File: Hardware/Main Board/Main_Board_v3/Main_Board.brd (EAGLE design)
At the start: 105.4 x 84.8 mm, 69 parts, among them IC1 MBED_MICROCONTROLLER, IC2 NE555, Q1 BS170, Q2 BS170, Q3 IRF3704L-V, Q4 IRF3704L-V, Q5 BS170, Q6 IRF3704L-V, Q7 BS170, Q8 IRF3704L-V

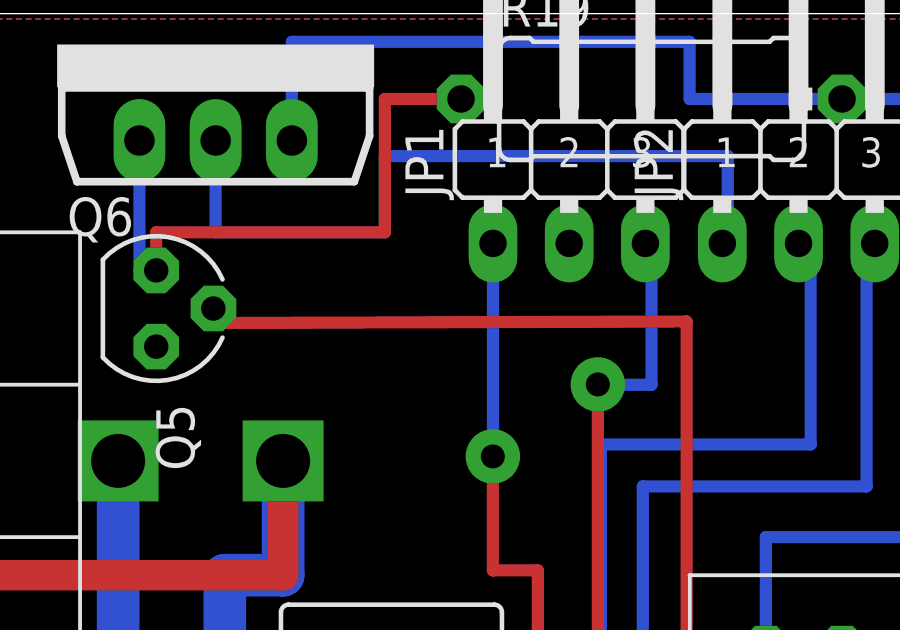
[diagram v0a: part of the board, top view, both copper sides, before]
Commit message: Board Layouts done for DC Current and AC Board
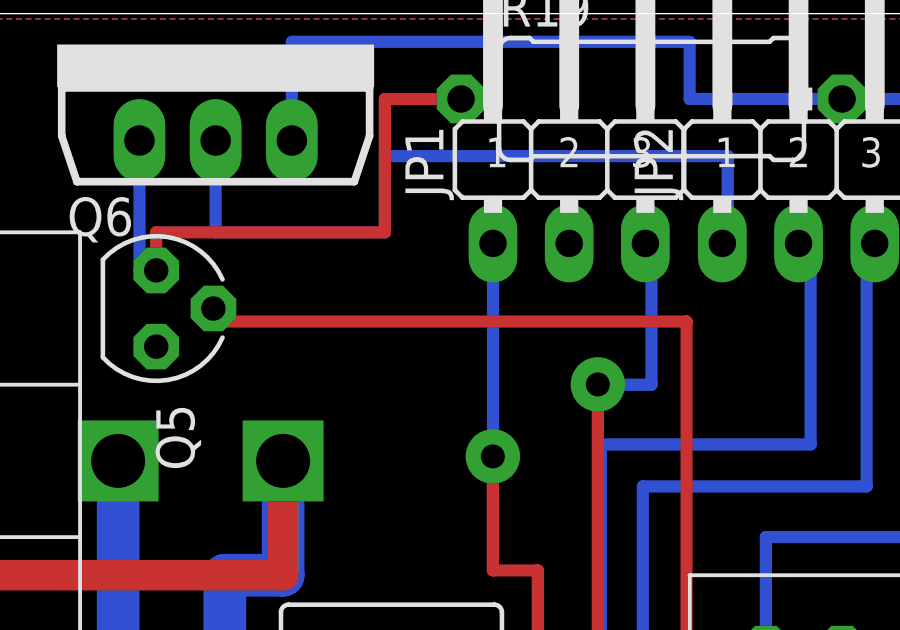
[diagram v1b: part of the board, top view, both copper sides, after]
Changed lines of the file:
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@@
 <wire x1="62.23" y1="53.34" x2="35.4584" y2="53.3908" width="0.4064" layer="1"/>
 <wire x1="35.4584" y1="53.3908" x2="35.4584" y2="74.4982" width="0.4064" layer="1"/>
-<wire x1="35.4584" y1="74.4982" x2="19.7358" y2="74.4474" width="0.4064" layer="1"/>
-<wire x1="19.7358" y1="74.4474" x2="19.7358" y2="74.9808" width="0.4064" layer="1"/>
-<wire x1="19.7358" y1="74.9808" x2="19.685" y2="74.93" width="0" layer="19" extent="1-1"/>
+<wire x1="35.4584" y1="74.4982" x2="19.685" y2="74.4982" width="0.4064" layer="1"/>
+<wire x1="19.685" y1="74.4982" x2="19.685" y2="74.93" width="0.4064" layer="1"/>
 </signal>
 <signal name="N$7">
